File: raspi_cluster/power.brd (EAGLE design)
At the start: 28.9 x 34.3 mm, 5 parts

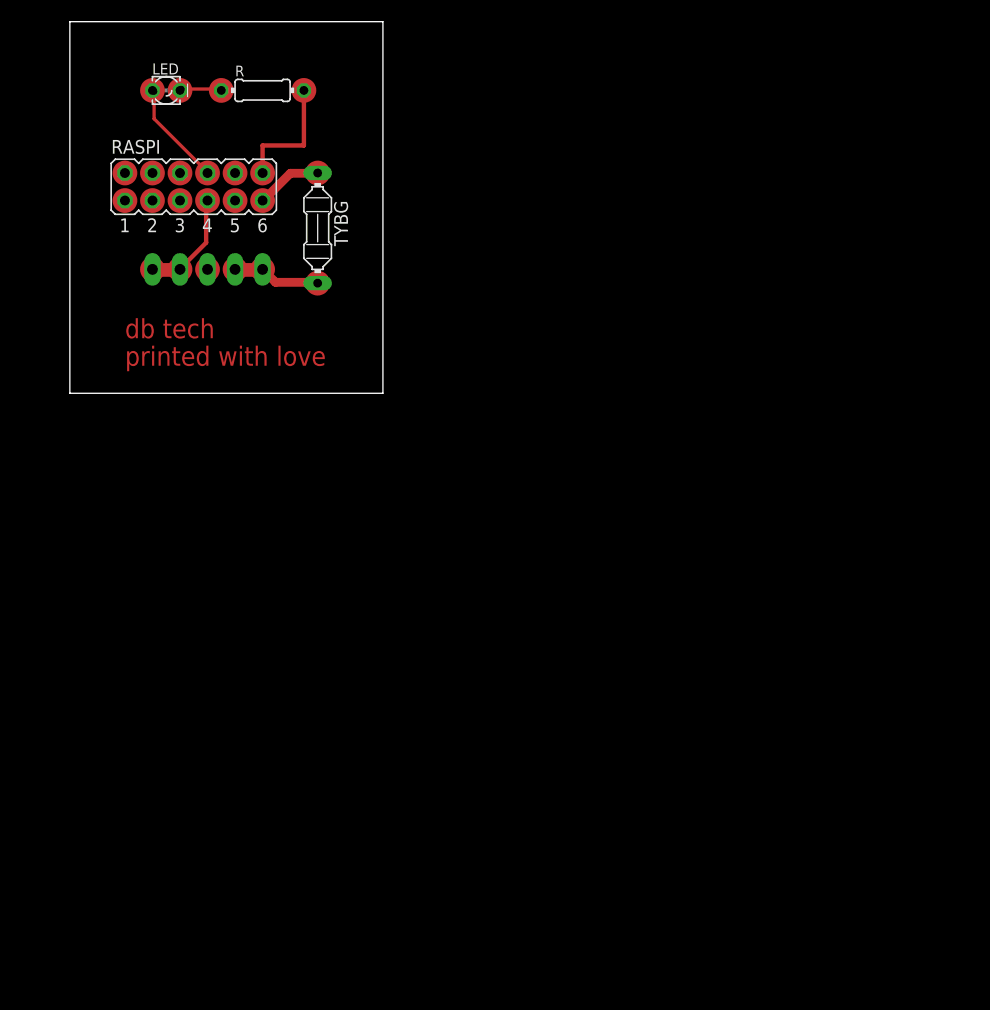
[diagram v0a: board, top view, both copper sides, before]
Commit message: made the printable pcb design
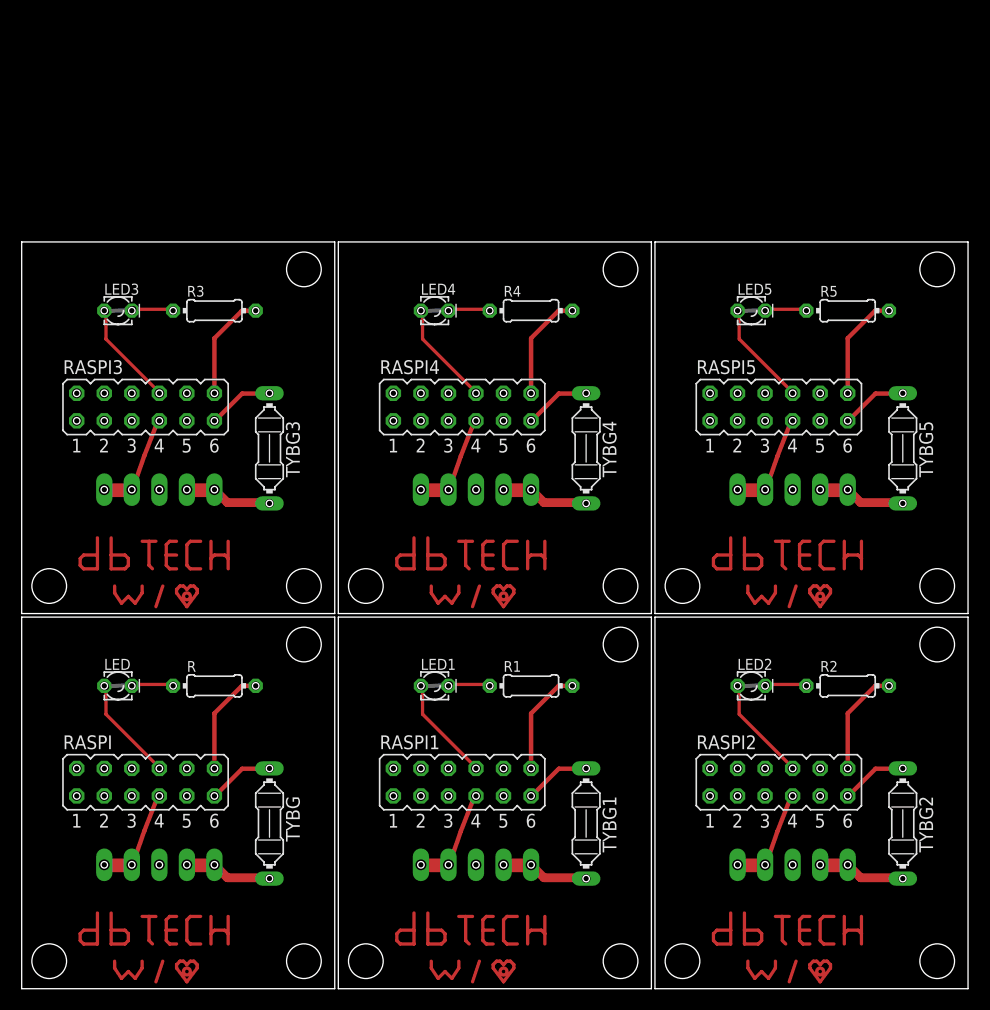
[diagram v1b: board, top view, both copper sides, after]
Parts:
- added 5V1, 5V2, 5V3, 5V4, 5V5: 22-23-2051, con-molex:22-23-2051
- added LED1, LED2, LED3, LED4, LED5: (no value), eagle-ltspice:LED_LD260
- added R1, R2, R3, R4, R5: (no value), resistor:0204/7
- added RASPI1, RASPI2, RASPI3, RASPI4, RASPI5: (no value), jumper:JP6Q
- added TYBG1, TYBG2, TYBG3, TYBG4, TYBG5: FUSEPICOFUSE, fuse:PICOFUSE
- moved TYBG 55.1 mm to (18.4, 11.1)
- moved 5V 55.1 mm to (8.26, 7.30)
- moved LED 55.1 mm to (4.45, 23.8)
- moved R 55.1 mm to (13.3, 23.8)
- moved RASPI 55.1 mm to (6.99, 14.9)
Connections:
- new net N$10: RASPI1.11, TYBG1.1
- new net N$11: 5V1.4, 5V1.5, RASPI1.7
- new net N$12: R1.2, RASPI1.12
- new net N$13: 5V2.1, 5V2.2, TYBG2.2
- new net N$14: LED2.A, R2.1
- new net N$15: LED2.K, RASPI2.8
- new net N$16: RASPI2.11, TYBG2.1
- new net N$17: 5V2.4, 5V2.5, RASPI2.7
- new net N$18: R2.2, RASPI2.12
- new net N$19: 5V3.1, 5V3.2, TYBG3.2
- new net N$20: LED3.A, R3.1
- new net N$21: LED3.K, RASPI3.8
- new net N$22: RASPI3.11, TYBG3.1
- new net N$23: 5V3.4, 5V3.5, RASPI3.7
- new net N$24: R3.2, RASPI3.12
- new net N$25: 5V4.1, 5V4.2, TYBG4.2
- new net N$26: LED4.A, R4.1
- new net N$27: LED4.K, RASPI4.8
- new net N$28: RASPI4.11, TYBG4.1
- new net N$29: 5V4.4, 5V4.5, RASPI4.7
- new net N$30: R4.2, RASPI4.12
- new net N$31: 5V5.1, 5V5.2, TYBG5.2
- new net N$32: LED5.A, R5.1
- new net N$33: LED5.K, RASPI5.8
- new net N$34: RASPI5.11, TYBG5.1
- new net N$35: 5V5.4, 5V5.5, RASPI5.7
- new net N$36: R5.2, RASPI5.12
- new net N$7: 5V1.1, 5V1.2, TYBG1.2
- new net N$8: LED1.A, R1.1
- new net N$9: LED1.K, RASPI1.8
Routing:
- net N$33: track 0.00 -> 11.7 mm, vias 0 -> 1
- net N$15: track 0.00 -> 11.7 mm, vias 0 -> 1
- net N$9: track 0.00 -> 11.7 mm, vias 0 -> 1
- net N$27: track 0.00 -> 11.7 mm, vias 0 -> 1
- net N$21: track 0.00 -> 11.7 mm, vias 0 -> 1
- net N$36: track 0.00 -> 9.94 mm
- net N$24: track 0.00 -> 9.94 mm
- net N$18: track 0.00 -> 9.94 mm
- net N$30: track 0.00 -> 9.94 mm
- net N$12: track 0.00 -> 9.94 mm
- net N$17: track 0.00 -> 9.36 mm
- net N$35: track 0.00 -> 9.36 mm
- net N$11: track 0.00 -> 9.36 mm
- net N$29: track 0.00 -> 9.36 mm
- net N$23: track 0.00 -> 9.36 mm
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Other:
- board size 28.9 x 34.3 mm -> 87.3 x 68.9 mm
- board text removed: "db tech"
- board text removed: "printed with love"
